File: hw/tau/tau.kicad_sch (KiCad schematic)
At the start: 46 parts, among them J1 USB_B, J2 AudioIn, J3 AudioOut, SW1 SW_bypass, SW2 SW_cahnnel_up, SW3 SW_midi, SW4 SW_sustain, SW5 SW_channel_down, U1 MCP6002-xMS

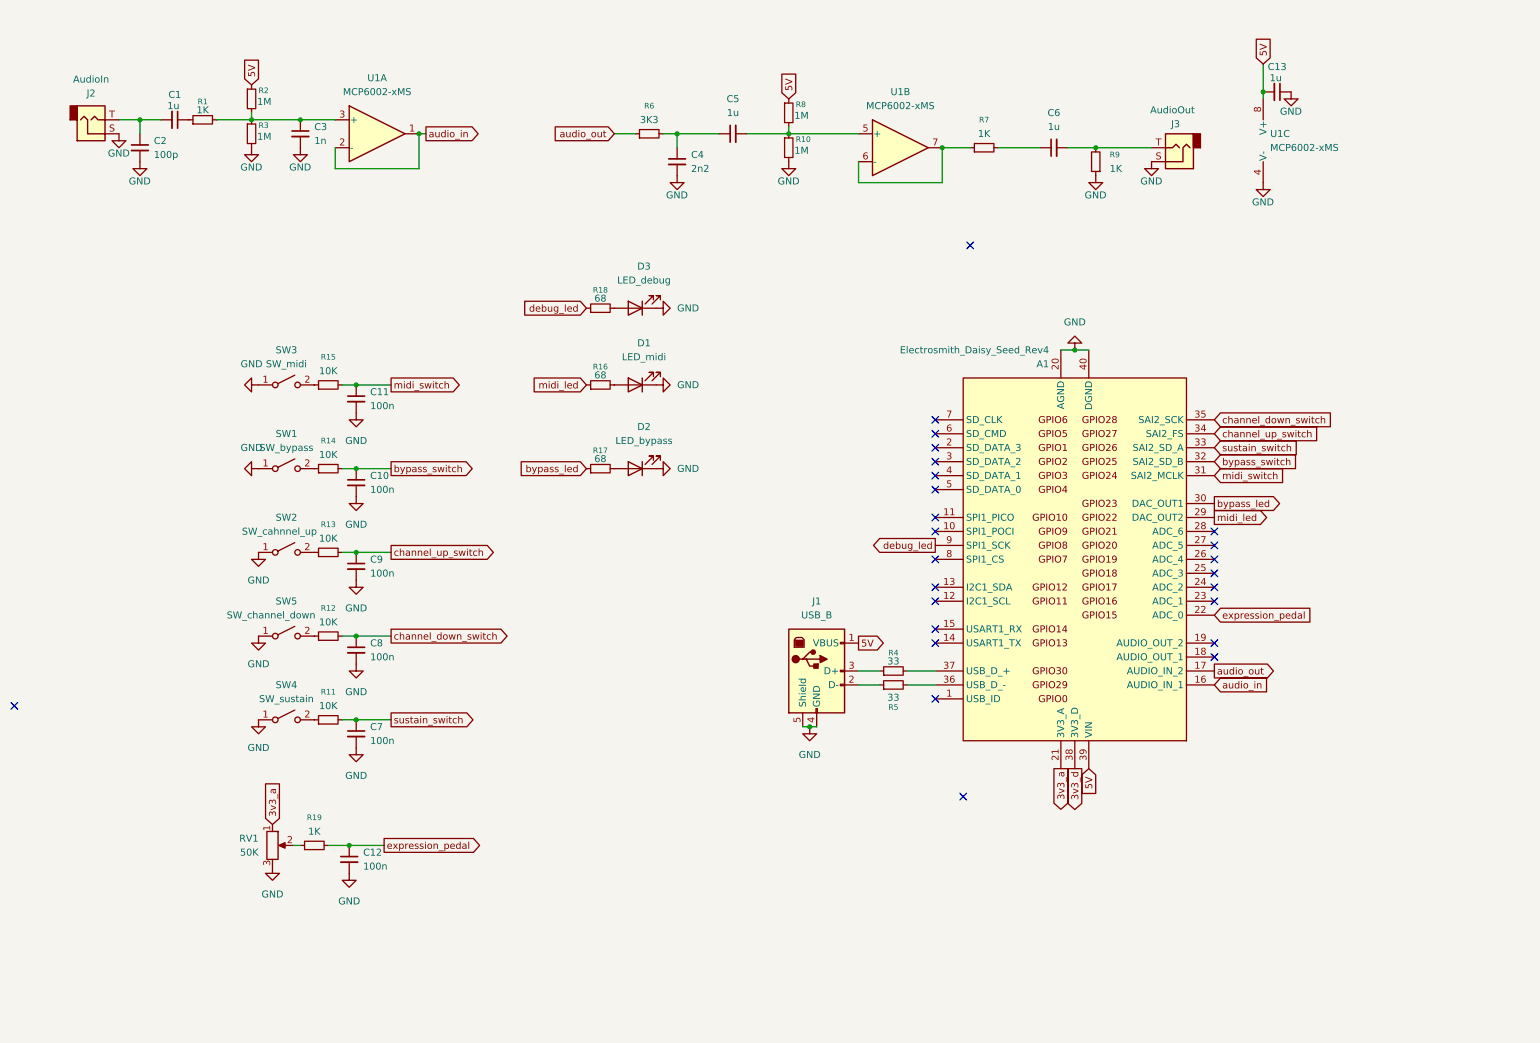
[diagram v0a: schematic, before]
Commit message: god is dead and we killed him. new pcb.
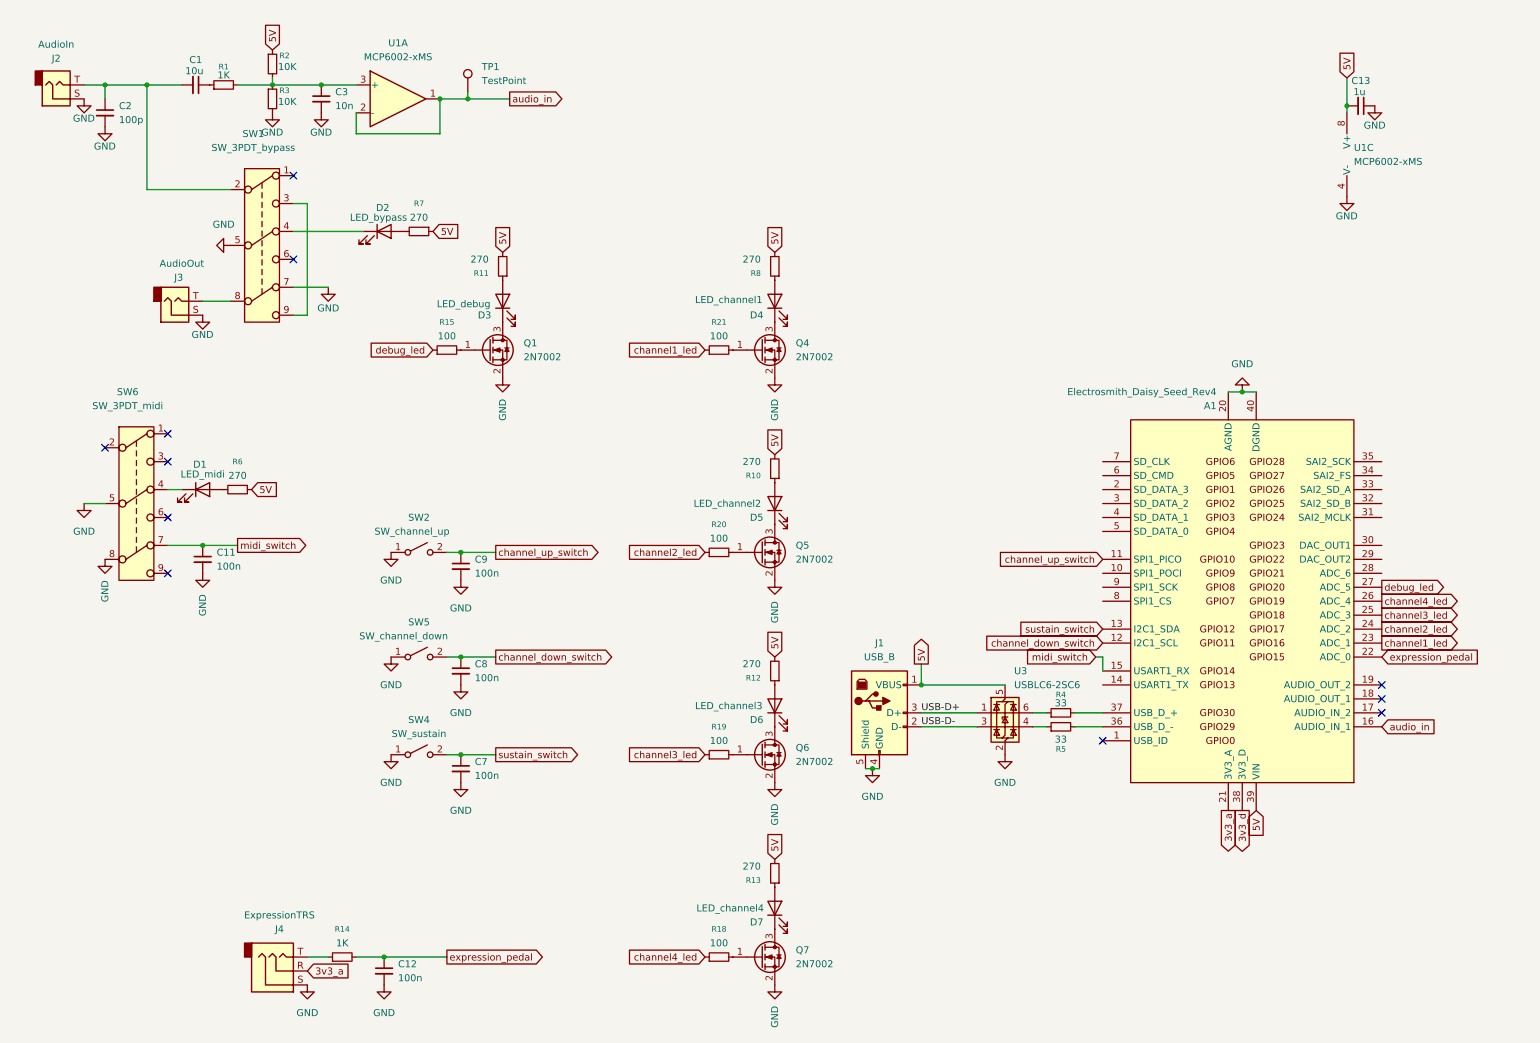
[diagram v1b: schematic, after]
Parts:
- removed C10: 100n, Capacitor_SMD:C_0603_1608Metric_Pad1.08x0.95mm_HandSolder, symbol Device:C_Small
- removed C4: 2n2, Capacitor_SMD:C_0603_1608Metric_Pad1.08x0.95mm_HandSolder, symbol Device:C_Small
- removed C5, C6: 1u, Capacitor_SMD:C_0603_1608Metric_Pad1.08x0.95mm_HandSolder, symbol Device:C_Small
- removed R16, R17: 68, Resistor_SMD:R_0603_1608Metric_Pad0.98x0.95mm_HandSolder, symbol Device:R_Small
- removed R9: 1K, Resistor_SMD:R_0603_1608Metric_Pad0.98x0.95mm_HandSolder, symbol Device:R_Small
- removed RV1: 50K, Connector_PinHeader_2.54mm:PinHeader_1x03_P2.54mm_Vertical, symbol Device:R_Potentiometer
- removed SW1: SW_bypass, Connector_PinHeader_2.54mm:PinHeader_1x02_P2.54mm_Vertical, symbol Switch:SW_SPST
- removed SW3: SW_midi, Connector_PinHeader_2.54mm:PinHeader_1x02_P2.54mm_Vertical, symbol Switch:SW_SPST
- removed unit 2 of U1
- added D4: LED_channel1, Connector_JST:JST_XH_B2B-XH-A_1x02_P2.50mm_Vertical, symbol Device:LED
- added D5: LED_channel2, Connector_JST:JST_XH_B2B-XH-A_1x02_P2.50mm_Vertical, symbol Device:LED
- added D6: LED_channel3, Connector_JST:JST_XH_B2B-XH-A_1x02_P2.50mm_Vertical, symbol Device:LED
- added D7: LED_channel4, Connector_JST:JST_XH_B2B-XH-A_1x02_P2.50mm_Vertical, symbol Device:LED
- added J4: ExpressionTRS, Connector_Audio:Jack_6.35mm_Neutrik_NRJ6HH-AU_Horizontal, symbol Connector_Audio:AudioJack3
- added Q1, Q4, Q5, Q6, Q7: 2N7002, Package_TO_SOT_SMD:SOT-23, symbol Transistor_FET:2N7002
- added R20, R21: 100, Resistor_SMD:R_0805_2012Metric_Pad1.20x1.40mm_HandSolder, symbol Device:R_Small
- added SW1: SW_3PDT_bypass, 3pdt:SW_3PDT, symbol 3pdt:3pdt
- added SW6: SW_3PDT_midi, 3pdt:SW_3PDT, symbol 3pdt:3pdt
- added TP1: TestPoint, Connector_Pin:Pin_D1.0mm_L10.0mm_LooseFit, symbol Connector:TestPoint
- added U3: USBLC6-2SC6, Package_TO_SOT_SMD:SOT-23-6, symbol Power_Protection:USBLC6-2SC6
- C1: value 1u -> 10u; footprint Capacitor_SMD:C_0603_1608Metric_Pad1.08x0.95mm_HandSolder -> Capacitor_SMD:C_0805_2012Metric_Pad1.18x1.45mm_HandSolder
- C11, C12, C13, C2, C7, C8, C9: footprint Capacitor_SMD:C_0603_1608Metric_Pad1.08x0.95mm_HandSolder -> Capacitor_SMD:C_0805_2012Metric_Pad1.18x1.45mm_HandSolder
- C3: value 1n -> 10n; footprint Capacitor_SMD:C_0603_1608Metric_Pad1.08x0.95mm_HandSolder -> Capacitor_SMD:C_0805_2012Metric_Pad1.18x1.45mm_HandSolder
- D1, D2: footprint Connector_PinHeader_2.54mm:PinHeader_1x02_P2.54mm_Vertical -> Connector_JST:JST_XH_B2B-XH-A_1x02_P2.50mm_Vertical
- R1, R4, R5: footprint Resistor_SMD:R_0603_1608Metric_Pad0.98x0.95mm_HandSolder -> Resistor_SMD:R_0805_2012Metric_Pad1.20x1.40mm_HandSolder
- R10, R8: value 1M -> 270; footprint Resistor_SMD:R_0603_1608Metric_Pad0.98x0.95mm_HandSolder -> Resistor_SMD:R_0805_2012Metric_Pad1.20x1.40mm_HandSolder
- R11, R12, R13: value 10K -> 270; footprint Resistor_SMD:R_0603_1608Metric_Pad0.98x0.95mm_HandSolder -> Resistor_SMD:R_0805_2012Metric_Pad1.20x1.40mm_HandSolder
- R14: value 10K -> 1K; footprint Resistor_SMD:R_0603_1608Metric_Pad0.98x0.95mm_HandSolder -> Resistor_SMD:R_0805_2012Metric_Pad1.20x1.40mm_HandSolder
- R15: value 10K -> 100; footprint Resistor_SMD:R_0603_1608Metric_Pad0.98x0.95mm_HandSolder -> Resistor_SMD:R_0805_2012Metric_Pad1.20x1.40mm_HandSolder
- R18: value 68 -> 100; footprint Resistor_SMD:R_0603_1608Metric_Pad0.98x0.95mm_HandSolder -> Resistor_SMD:R_0805_2012Metric_Pad1.20x1.40mm_HandSolder
- R19: value 1K -> 100; footprint Resistor_SMD:R_0603_1608Metric_Pad0.98x0.95mm_HandSolder -> Resistor_SMD:R_0805_2012Metric_Pad1.20x1.40mm_HandSolder
- R2, R3: value 1M -> 10K; footprint Resistor_SMD:R_0603_1608Metric_Pad0.98x0.95mm_HandSolder -> Resistor_SMD:R_0805_2012Metric_Pad1.20x1.40mm_HandSolder
- R6: value 3K3 -> 270; footprint Resistor_SMD:R_0603_1608Metric_Pad0.98x0.95mm_HandSolder -> Resistor_SMD:R_0805_2012Metric_Pad1.20x1.40mm_HandSolder
- R7: value 1K -> 270; footprint Resistor_SMD:R_0603_1608Metric_Pad0.98x0.95mm_HandSolder -> Resistor_SMD:R_0805_2012Metric_Pad1.20x1.40mm_HandSolder
- SW2: value SW_cahnnel_up -> SW_channel_up
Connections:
- net 3v3_a: now also J4.R
- net 5V: now also R10.2, R11.2, R12.2, R13.2, R6.1, R7.1, R8.2, U3.5 (VBUS); no longer R8.1
- net GND: now also J4.S, Q1.2 (S), Q4.2 (S), Q5.2 (S), Q6.2 (S), Q7.2 (S), SW1.5, SW1.7, SW6.5, SW6.8, U3.2 (GND); no longer D1.1 (K), D2.1 (K), D3.1 (K), R10.2
- net audio_in: now also TP1.1
- net channel_down_switch: now also A1.12 (I2C1_SCL), SW5.2 (B); no longer A1.35 (SAI2_SCK), R12.2
- net channel_up_switch: now also A1.11 (SPI1_PICO), SW2.2 (B); no longer A1.34 (SAI2_FS), R13.2
- net debug_led: now also A1.27 (ADC_5), R15.1; no longer A1.9 (SPI1_SCK), R18.1
- net expression_pedal: now also R14.2; no longer R19.2
- net midi_switch: now also A1.15 (USART1_RX), SW6.7; no longer A1.31 (SAI2_MCLK), R15.2
- net sustain_switch: now also A1.13 (I2C1_SDA), SW4.2 (B); no longer A1.33 (SAI2_SD_A), R11.2
- net at J3.T: now also SW1.8
- net at R6.2: now also D1.2 (A)
- net at R12.1: now also D6.2 (A); no longer SW5.2 (B)
- net at R10.1: now also D5.2 (A); no longer R8.2
- net at R4.1: now also U3.6 (I/O1); no longer J1.3 (D+)
- net at D2.2 (A): now also R7.2
- net at C1.2, C2.1, J2.T: now also SW1.2
- net at D3.2 (A): now also R11.1; no longer R18.2
- net at R5.1: now also U3.4 (I/O2); no longer J1.2 (D-)
- net at R13.1: now also D7.2 (A); no longer SW2.2 (B)
- net channel3_led: now reaches R19.1
- net channel3_led: now also A1.25 (ADC_3)
- net at R14.1: now also J4.T
- net channel1_led: now reaches A1.23 (ADC_1)
- net channel1_led: now also R21.1
- net channel2_led: now reaches A1.24 (ADC_2)
- net channel2_led: now also R20.1
- net channel4_led: now reaches A1.26 (ADC_4)
- net channel4_led: now also R18.1
- net audio_out: no longer names the net of A1.17 (AUDIO_IN_2)
- net audio_out: no longer R6.1
- net bypass_led: no longer names the net of A1.30 (DAC_OUT1)
- net bypass_switch: no longer names the net of A1.32 (SAI2_SD_B)
- net bypass_switch: no longer R14.2
- net midi_led: no longer names the net of A1.29 (DAC_OUT2)
- new net: Q4.1 (G), R21.2
- new net: D4.1 (K), Q4.3 (D)
- new net: Q1.1 (G), R15.2
- new net: D3.1 (K), Q1.3 (D)
- new net: D1.1 (K), SW6.4
- new net: D6.1 (K), Q6.3 (D)
- new net: D4.2 (A), R8.1
- new net: Q7.1 (G), R18.2
- new net: SW1.3, SW1.9
- new net: D2.1 (K), SW1.4
- new net: D7.1 (K), Q7.3 (D)
- new net: Q6.1 (G), R19.2
- new net: Q5.1 (G), R20.2
- new net: D5.1 (K), Q5.3 (D)
- new net USB-D+: J1.3 (D+), U3.1 (I/O1)
- new net USB-D-: J1.2 (D-), U3.3 (I/O2)
- no-connect marks 25 -> 11
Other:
- moved on the sheet: A1, C1, C11, C12, C13, C2, C3, C7, C8, C9, D3, J1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

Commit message: hardware_final_final
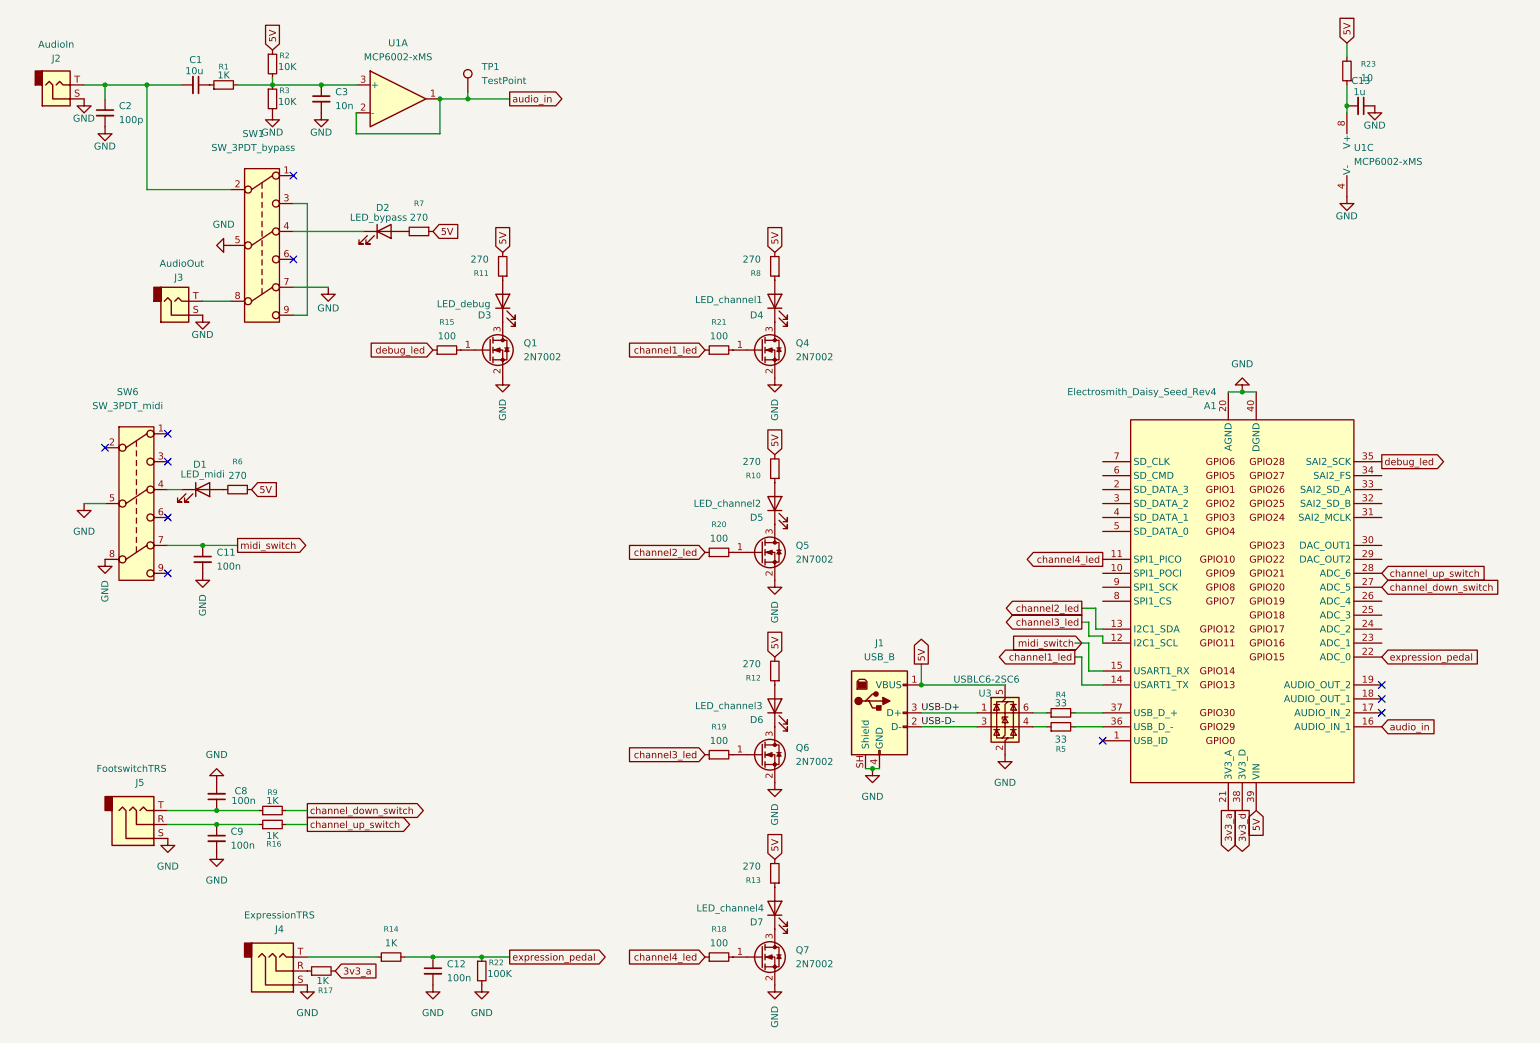
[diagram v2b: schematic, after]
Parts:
- removed C7: 100n, Capacitor_SMD:C_0805_2012Metric_Pad1.18x1.45mm_HandSolder, symbol Device:C_Small
- removed SW2: SW_channel_up, Connector_PinHeader_2.54mm:PinHeader_1x02_P2.54mm_Vertical, symbol Switch:SW_SPST
- removed SW4: SW_sustain, Connector_PinHeader_2.54mm:PinHeader_1x02_P2.54mm_Vertical, symbol Switch:SW_SPST
- removed SW5: SW_channel_down, Connector_PinHeader_2.54mm:PinHeader_1x02_P2.54mm_Vertical, symbol Switch:SW_SPST
- added J5: FootswitchTRS, Connector_Audio:Jack_6.35mm_Neutrik_NRJ6HH-AU_Horizontal, symbol Connector_Audio:AudioJack3
- added R16, R17, R9: 1K, Resistor_SMD:R_0805_2012Metric_Pad1.20x1.40mm_HandSolder, symbol Device:R_Small
- added R22: 100K, Resistor_SMD:R_0805_2012Metric_Pad1.20x1.40mm_HandSolder, symbol Device:R_Small
- added R23: 10, Resistor_SMD:R_0805_2012Metric_Pad1.20x1.40mm_HandSolder, symbol Device:R_Small
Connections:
- net sustain_switch is gone; now on net channel2_led: A1.13 (I2C1_SDA)
- net 3v3_a: now also R17.2; no longer J4.R
- net 5V: now also R23.2; no longer C13.2, U1.8 (V+)
- net GND: now also J1.SH (Shield), J5.S, R22.2; no longer J1.5 (Shield)
- net channel1_led: now also A1.14 (USART1_TX); no longer A1.23 (ADC_1)
- net channel2_led: no longer A1.24 (ADC_2)
- net channel3_led: now also A1.12 (I2C1_SCL); no longer A1.25 (ADC_3)
- net channel4_led: now also A1.11 (SPI1_PICO); no longer A1.26 (ADC_4)
- net channel_down_switch: now also A1.27 (ADC_5), R9.2; no longer A1.12 (I2C1_SCL), C8.1
- net channel_up_switch: now also A1.28 (ADC_6), R16.2; no longer A1.11 (SPI1_PICO), C9.1
- net debug_led: now also A1.35 (SAI2_SCK); no longer A1.27 (ADC_5)
- net expression_pedal: now also R22.1
- new net: C8.1, J5.T, R9.1
- new net: J4.R, R17.1
- new net: C13.2, R23.1, U1.8 (V+)
- new net: C9.1, J5.R, R16.1
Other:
- moved on the sheet: C12, C8, C9, R14
